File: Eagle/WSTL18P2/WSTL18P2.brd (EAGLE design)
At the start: 23.5 x 23.5 mm, 24 parts, among them CON1 1X6CONN-1.27-ROUND, CON2 1X6CONN-1.27-ROUND, CON3 1X6CONN-1.27-ROUND, CON4 1X6CONN-1.27-ROUND, T1 ABS07AIG

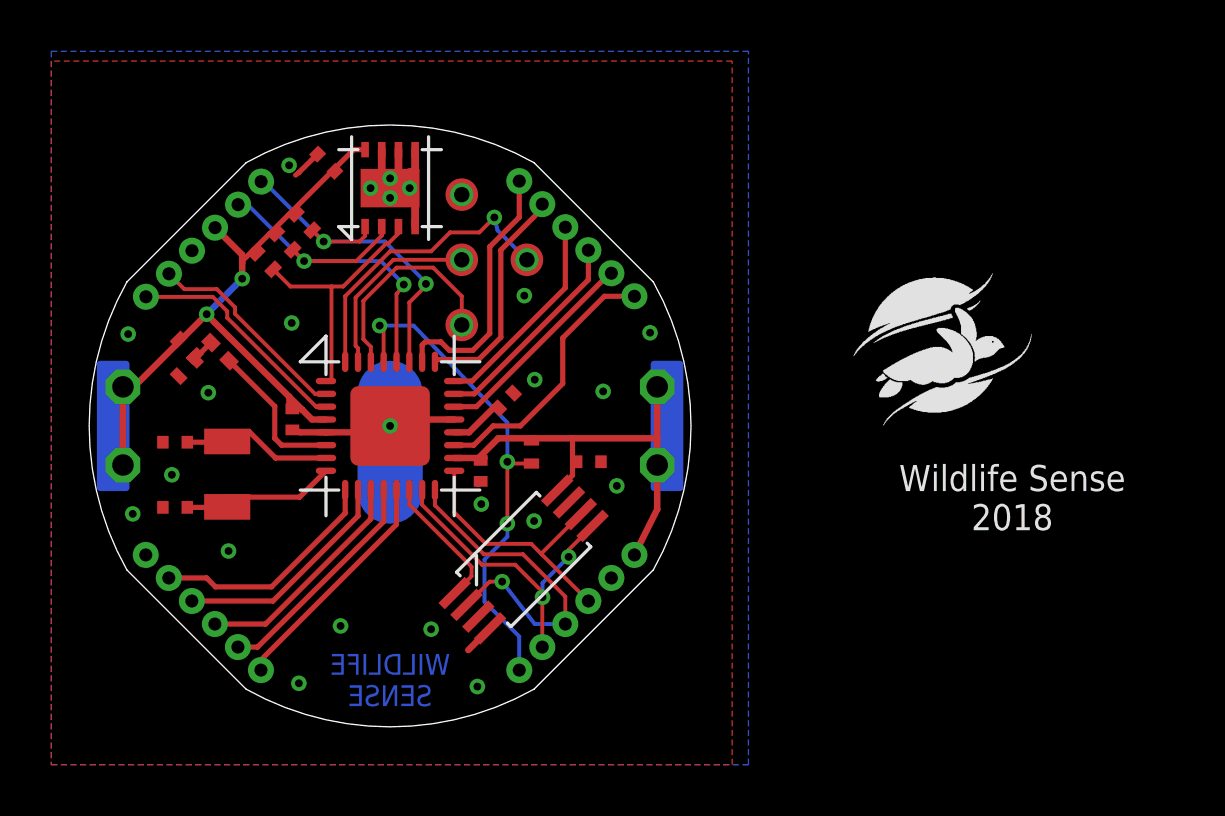
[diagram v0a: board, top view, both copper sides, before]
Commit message: Final corrections for WSTL18P2
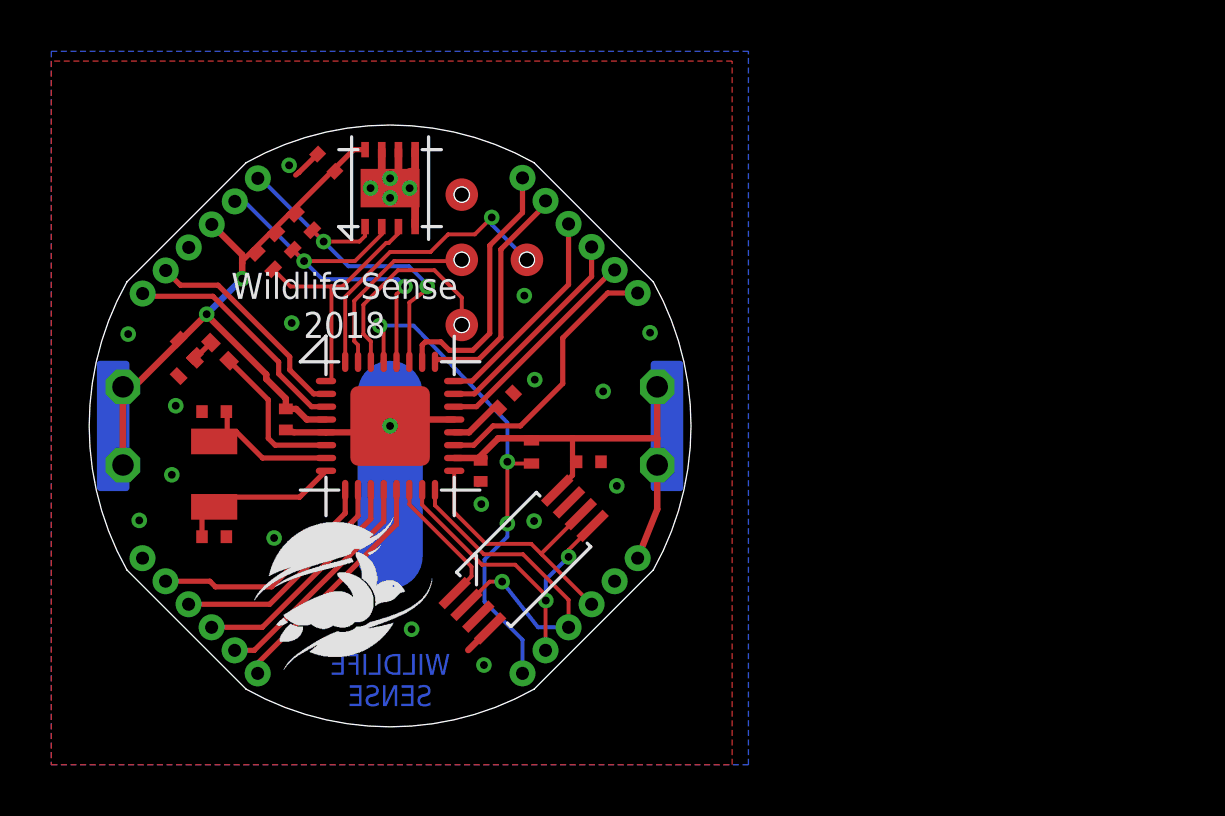
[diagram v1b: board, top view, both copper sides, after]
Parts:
- moved C6 1.94 mm to (6.35, 13.8)
- moved C7 1.90 mm to (6.35, 8.89), turned to 0 degrees
- moved T1 0.51 mm to (6.35, 11.3)
- moved C1 0.25 mm to (9.14, 13.5)
- moved CON3 0.18 mm to (22.9, 18.4)
- moved CON2 0.18 mm to (3.56, 8.05)
- moved CON1 0.18 mm to (22.9, 8.05)
- moved CON4 0.18 mm to (8.05, 22.9)
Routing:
- net N$1: track 6.22 -> 6.80 mm
- net GND: track 14.7 -> 15.0 mm, vias 24 -> 21
- net RXD0: track 8.45 -> 8.25 mm, vias 1 -> 0
- net PD2: track 11.8 -> 11.7 mm, vias 2 -> 1
- net TXD0: vias 1 -> 0

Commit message: Approved and cleared design rules checks
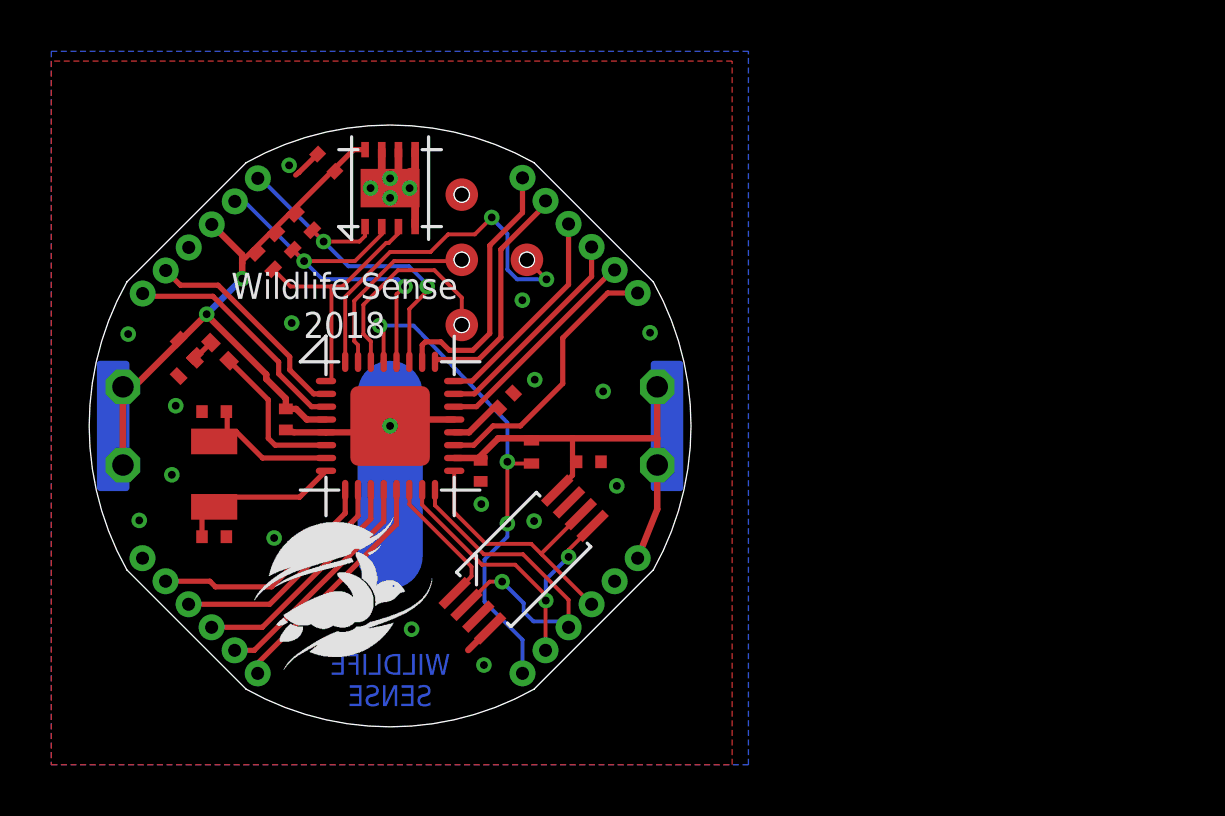
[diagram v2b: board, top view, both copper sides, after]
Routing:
- net PD2: track 11.7 -> 14.6 mm, vias 1 -> 2
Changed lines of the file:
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@@
 <wire x1="14.8336" y1="19.0754" x2="14.4526" y2="19.0754" width="0.254" layer="51"/>
 <wire x1="14.224" y1="19.4564" x2="13.9446" y2="19.4564" width="0.2032" layer="51"/>
-<wire x1="14.1478" y1="18.5166" x2="13.97" y2="18.3388" width="0.254" layer="51"/>
+<wire x1="14.1478" y1="18.3896" x2="13.97" y2="18.2118" width="0.254" layer="51"/>
 <wire x1="10.7442" y1="19.9644" x2="10.4648" y2="19.9644" width="0.254" layer="51"/>
 <wire x1="13.9954" y1="19.0754" x2="14.224" y2="18.8468" width="0.254" layer="51"/>
@@
 <wire x1="8.1534" y1="22.86" x2="8.0518" y2="22.86" width="0.1524" layer="16"/>
 <contactref element="MCU" pad="27"/>
-<wire x1="13.958" y1="15.708" x2="13.958" y2="18.022" width="0.1524" layer="1"/>
-<wire x1="13.958" y1="18.022" x2="14.7066" y2="18.5674" width="0.1524" layer="1"/>
-<wire x1="14.7066" y1="18.5674" x2="14.6558" y2="18.6436" width="0.1524" layer="1"/>
+<wire x1="13.958" y1="15.708" x2="13.958" y2="17.768" width="0.1524" layer="1"/>
 <wire x1="10.6172" y1="20.3962" x2="12.0142" y2="20.3962" width="0.1524" layer="1"/>
 <wire x1="12.0142" y1="20.3962" x2="12.233" y2="20.615" width="0.1524" layer="1"/>
@@
 <wire x1="13.9446" y1="19.431" x2="11.5824" y2="19.431" width="0.1524" layer="16"/>
 <wire x1="11.5824" y1="19.431" x2="10.6172" y2="20.3962" width="0.1524" layer="16"/>
+<wire x1="13.958" y1="17.768" x2="14.6558" y2="18.4658" width="0.1524" layer="1"/>
+<wire x1="14.6558" y1="18.4658" x2="14.6558" y2="18.6436" width="0.1524" layer="1"/>
 </signal>
 <signal name="SCL0" class="2">
@@
 <contactref element="CON2" pad="1"/>
 <via x="21.5138" y="14.5542" extent="1-16" drill="0.3048"/>
-<via x="18.4404" y="18.288" extent="1-16" drill="0.3048"/>
+<via x="18.3642" y="18.1102" extent="1-16" drill="0.3048"/>
 <via x="16.8656" y="3.8862" extent="1-16" drill="0.3048"/>
 <via x="14.0462" y="5.2832" extent="1-16" drill="0.3048"/>
@@
 <via x="9.271" y="23.368" extent="1-16" drill="0.3048"/>
 <contactref element="UART" pad="4"/>
-<wire x1="16.7386" y1="11.0454" x2="16.637" y2="10.922" width="0.2032" layer="1"/>
 <wire x1="10.382921875" y1="23.805475" x2="9.652" y2="23.0886" width="0.2032" layer="1"/>
 <wire x1="9.652" y1="23.0886" x2="9.525" y2="22.987" width="0.2032" layer="1"/>
@@
 <wire x1="18.3896" y1="8.2042" x2="16.8656" y2="8.2042" width="0.1524" layer="1"/>
 <wire x1="16.8656" y1="8.2042" x2="14.958" y2="10.1118" width="0.1524" layer="1"/>
-<wire x1="17.5768" y1="7.1374" x2="18.975478125" y2="5.357721875" width="0.1524" layer="16"/>
-<wire x1="18.975478125" y1="5.357721875" x2="20.165921875" y2="5.357721875" width="0.1524" layer="16"/>
 <wire x1="14.958" y1="10.708" x2="14.958" y2="10.1118" width="0.1524" layer="1"/>
 <wire x1="16.1876125" y1="6.23323125" x2="17.09178125" y2="7.1374" width="0.1524" layer="1"/>
 <wire x1="17.09178125" y1="7.1374" x2="17.5768" y2="7.1374" width="0.1524" layer="1"/>
+<wire x1="17.5768" y1="7.1374" x2="18.415" y2="6.2992" width="0.1524" layer="16"/>
+<wire x1="18.415" y1="6.2992" x2="18.415" y2="5.969" width="0.1524" layer="16"/>
+<wire x1="18.415" y1="5.969" x2="18.796" y2="5.588" width="0.1524" layer="16"/>
+<wire x1="18.796" y1="5.588" x2="19.93564375" y2="5.588" width="0.1524" layer="16"/>
+<wire x1="19.93564375" y1="5.588" x2="20.165921875" y2="5.357721875" width="0.1524" layer="16"/>
 </signal>
 <signal name="SCK0" class="2">
@@
 <wire x1="16.51" y1="20.6756" x2="17.1704" y2="21.336" width="0.1524" layer="1"/>
 <via x="17.1704" y="21.336" extent="1-16" drill="0.3048" shape="octagon"/>
-<wire x1="17.1704" y1="21.0566" x2="18.542" y2="19.685" width="0.1524" layer="16"/>
-<wire x1="17.1704" y1="21.0566" x2="17.1704" y2="21.336" width="0.1524" layer="16"/>
-<wire x1="18.542" y1="19.685" x2="18.542" y2="19.685" width="0" layer="19" extent="1-16"/>
+<via x="19.304" y="18.923" extent="1-16" drill="0.3048" shape="octagon"/>
+<wire x1="19.304" y1="18.923" x2="18.542" y2="19.685" width="0.1524" layer="1"/>
+<wire x1="17.1704" y1="21.336" x2="17.1704" y2="21.3106" width="0.1524" layer="16"/>
+<wire x1="17.1704" y1="21.3106" x2="17.78" y2="20.701" width="0.1524" layer="16"/>
+<wire x1="17.78" y1="20.701" x2="17.78" y2="19.304" width="0.1524" layer="16"/>
+<wire x1="17.78" y1="19.304" x2="18.161" y2="18.923" width="0.1524" layer="16"/>
+<wire x1="18.161" y1="18.923" x2="19.304" y2="18.923" width="0.1524" layer="16"/>
 </signal>
 <signal name="PE2">
